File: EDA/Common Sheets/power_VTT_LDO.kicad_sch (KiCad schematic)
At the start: 27 parts, among them J5 Conn_01x04, U10 AZ1117-2.85, U9 TLV62569DBV

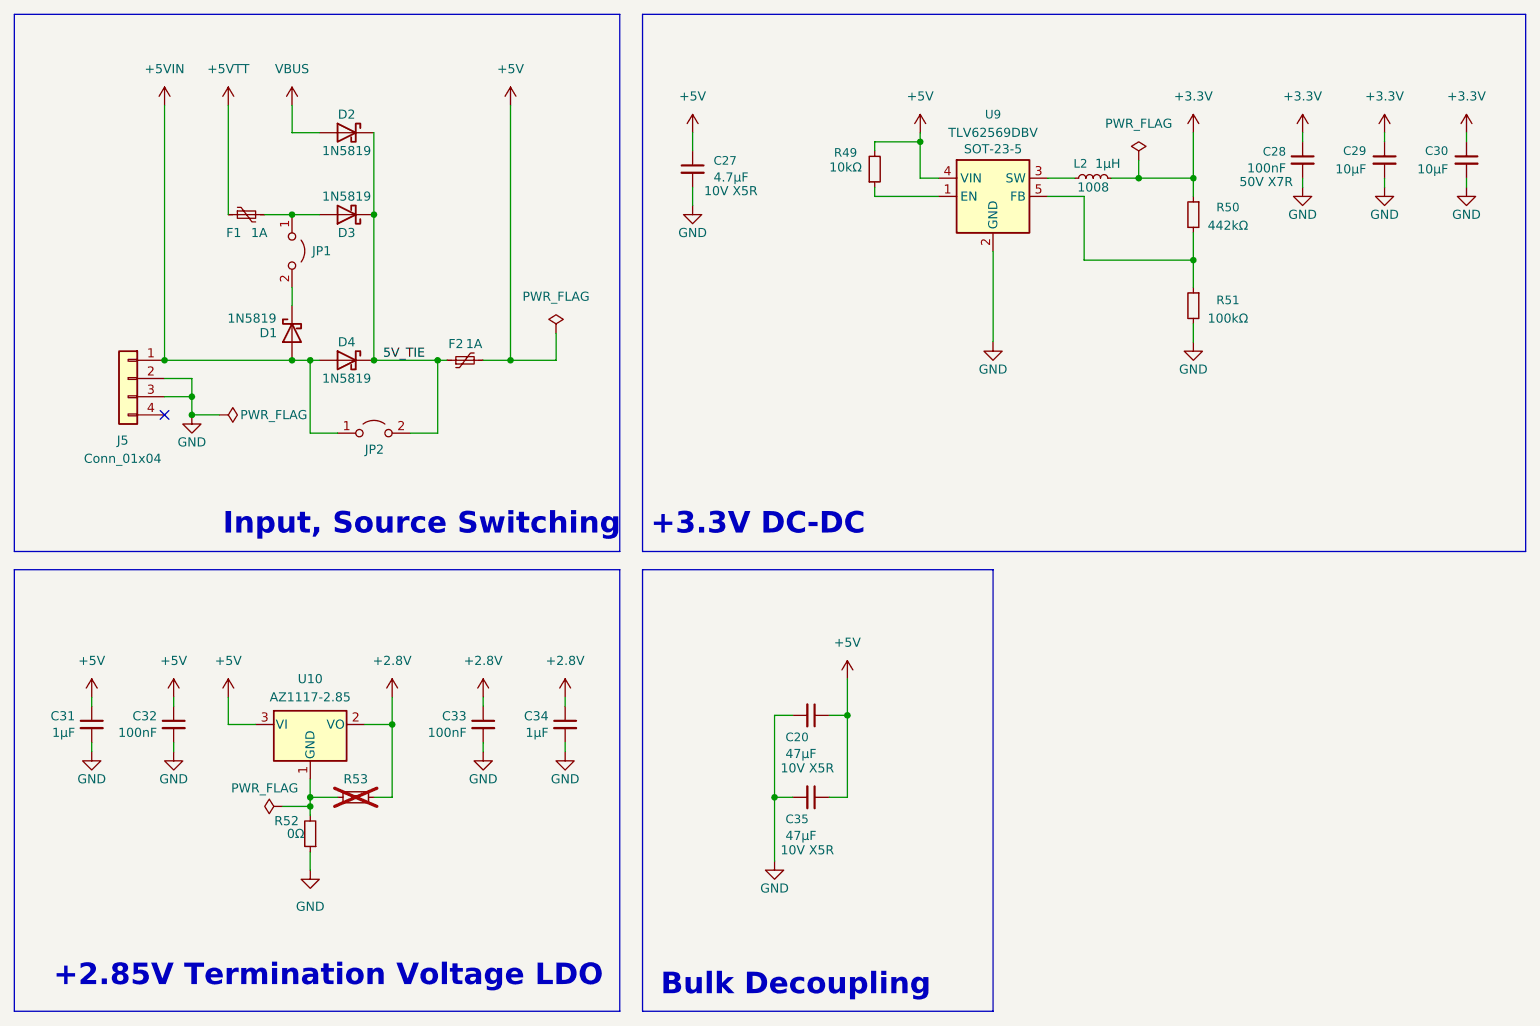
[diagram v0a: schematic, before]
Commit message: Resuming work
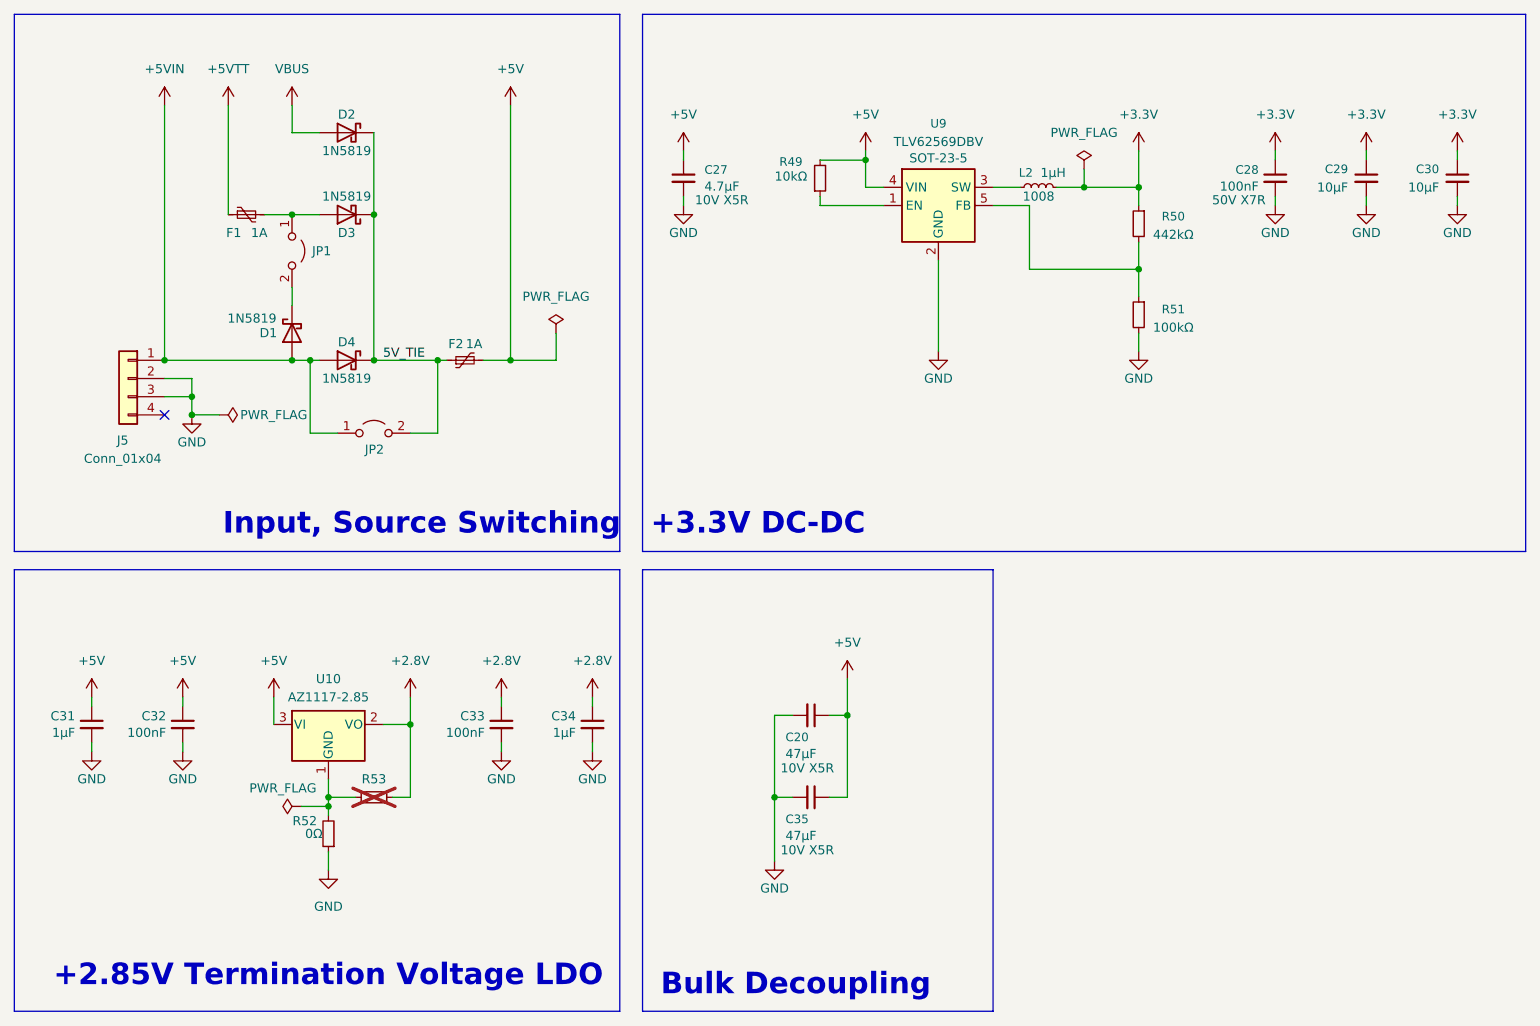
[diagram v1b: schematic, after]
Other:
- moved on the sheet: C27, C28, C29, C30, C32, C33, C34, L2, R49, R50, R51, R52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
